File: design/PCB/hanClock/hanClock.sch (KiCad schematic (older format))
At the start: 36 parts

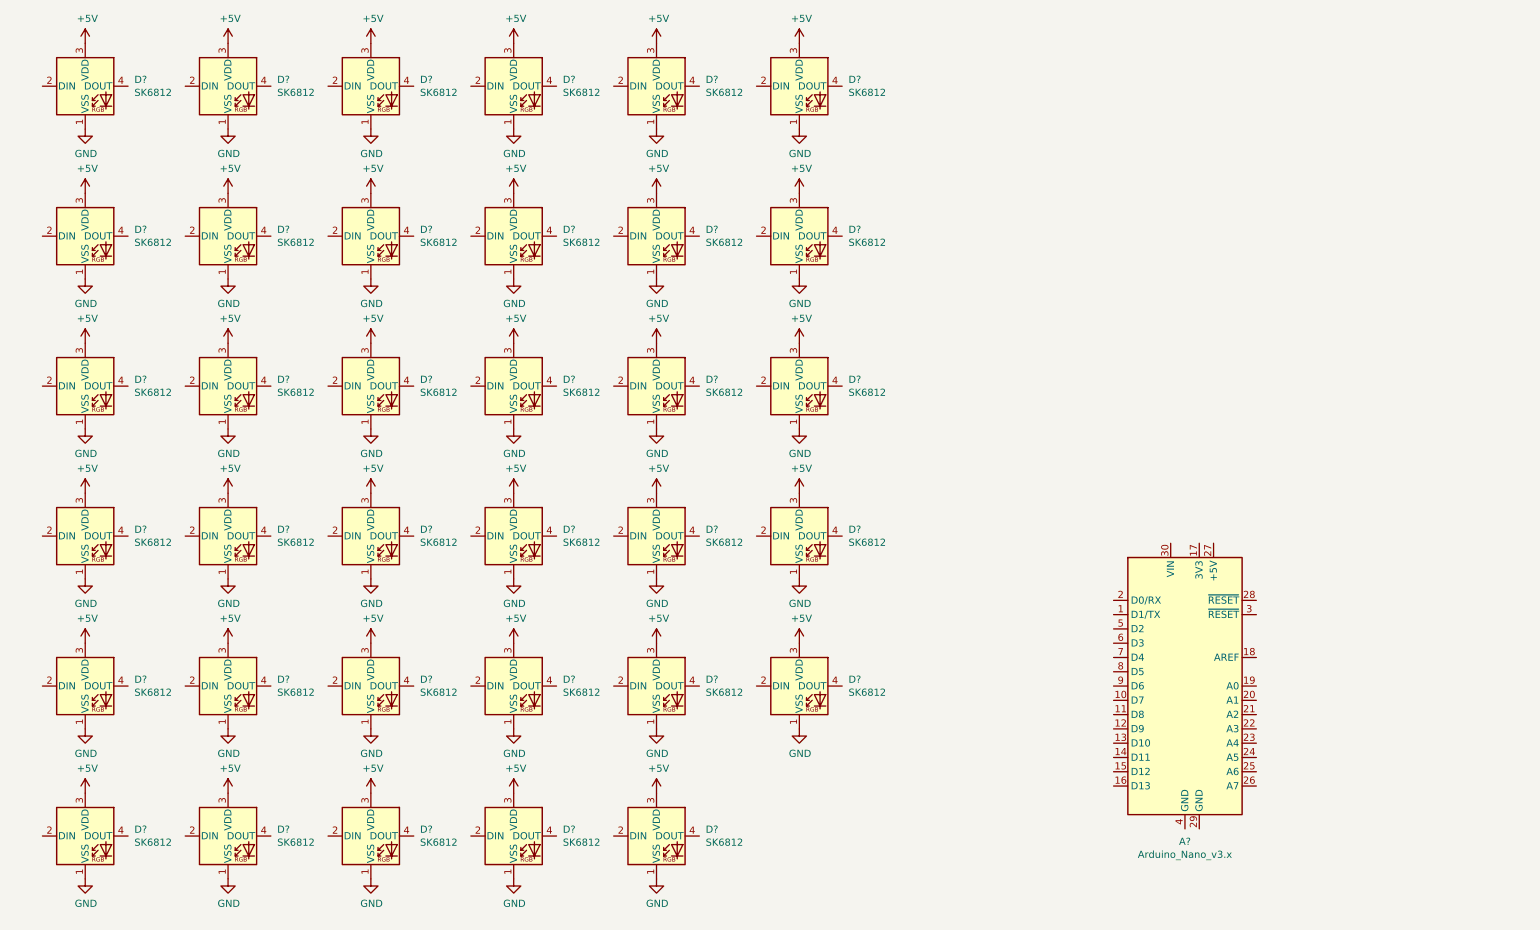
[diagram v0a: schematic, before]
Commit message: Finished design 커밋을 안 한 한참동안 PCB 다 만들고 외부 디자인도 다 해서 파일을 이렇게 저장했다.
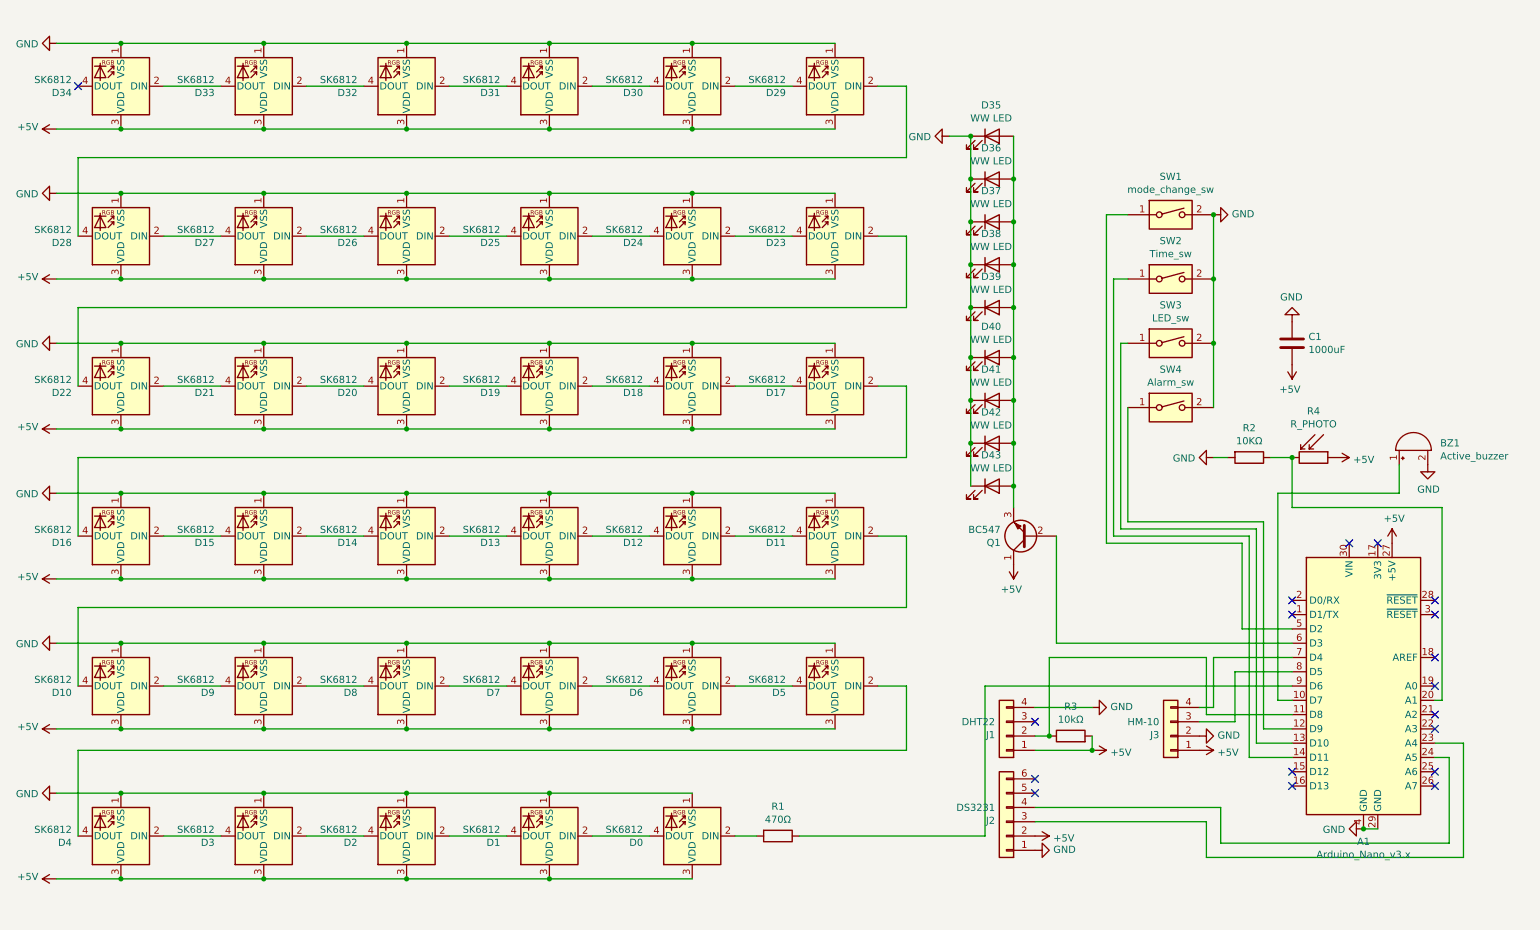
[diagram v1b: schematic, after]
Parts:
- added BZ1: Active_buzzer, parts:buzzer, symbol Device:Buzzer
- added C1: 1000uF, parts:C_K14, symbol Device:C
- added D35, D36, D37, D38, D39, D40, D41, D42, D43: WW LED, parts:3216LED, symbol Device:LED
- added J1: DHT22, parts:PinSocket_1x04_P2.54mm_Horizontal, symbol Connector_Generic:Conn_01x04
- added J2: DS3231, parts:PinSocket_1x06_P2.54mm_Horizontal, symbol Connector_Generic:Conn_01x06
- added J3: HM-10, Connector_PinSocket_2.54mm:PinSocket_1x04_P2.54mm_Vertical, symbol Connector_Generic:Conn_01x04
- added Q1: BC547, parts:BC547, symbol Device:Q_NPN_CBE
- added R1: 470Ω, Resistor_THT:R_Axial_DIN0207_L6.3mm_D2.5mm_P10.16mm_Horizontal, symbol Device:R
- added R2: 10KΩ, Resistor_THT:R_Axial_DIN0207_L6.3mm_D2.5mm_P10.16mm_Horizontal, symbol Device:R
- added R3: 10kΩ, Resistor_THT:R_Axial_DIN0207_L6.3mm_D2.5mm_P10.16mm_Horizontal, symbol Device:R
- added R4: R_PHOTO, Resistor_THT:R_Axial_DIN0204_L3.6mm_D1.6mm_P2.54mm_Vertical, symbol Device:R_PHOTO
- added SW1: mode_change_sw, parts:SMDbutton, symbol Switch:SW_DIP_x01
- added SW2: Time_sw, parts:KLT_SW, symbol Switch:SW_DIP_x01
- added SW3: LED_sw, parts:KLT_SW, symbol Switch:SW_DIP_x01
- added SW4: Alarm_sw, parts:KLT_SW, symbol Switch:SW_DIP_x01
- D0, D1, D10, D11, D12, D13, D14, D15, D16, D17, D18, D19, D2, D20, D21, D22, D23, D24, D25, D26, D27, D28, D29, D3, D30, D31, D32, D33, D34, D4, D5, D6, D7, D8, D9: renamed from D?; footprint LED_SMD:LED_SK6812_PLCC4_5.0x5.0mm_P3.2mm -> parts:LED_SK6812_PLCC4_5.0x5.0mm_P3.2mm
- gave numbers to parts that had none: 1
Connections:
- net +5V: now also A1.27 (+5V), C1.2, J1.1 (Pin_1), J2.2 (Pin_2), J3.1 (Pin_1), Q1.1 (C), R3.2, R4.1
- net GND: now also A1.29 (GND), A1.4 (GND), BZ1.2 (+), C1.1, D35.1 (K), D36.1 (K), D37.1 (K), D38.1 (K), D39.1 (K), D40.1 (K), D41.1 (K), D42.1 (K), D43.1 (K), J1.4 (Pin_4), J2.1 (Pin_1), J3.2 (Pin_2), R2.2, SW1.2, SW2.2, SW3.2, SW4.2
- net at D0.2 (DIN): now also R1.2
- net at D0.4 (DOUT): now also D1.2 (DIN)
- net at D34.2 (DIN): now also D33.4 (DOUT)
- net at D6.2 (DIN): now also D5.4 (DOUT)
- net at D6.4 (DOUT): now also D7.2 (DIN)
- net at D5.2 (DIN): now also D4.4 (DOUT)
- net at D2.2 (DIN): now also D1.4 (DOUT)
- net at D2.4 (DOUT): now also D3.2 (DIN)
- net at D8.2 (DIN): now also D7.4 (DOUT)
- net at D8.4 (DOUT): now also D9.2 (DIN)
- net at D12.2 (DIN): now also D11.4 (DOUT)
- net at D12.4 (DOUT): now also D13.2 (DIN)
- net at D11.2 (DIN): now also D10.4 (DOUT)
- net at D18.2 (DIN): now also D17.4 (DOUT)
- net at D18.4 (DOUT): now also D19.2 (DIN)
- net at D17.2 (DIN): now also D16.4 (DOUT)
- net at D14.2 (DIN): now also D13.4 (DOUT)
- net at D14.4 (DOUT): now also D15.2 (DIN)
- net at D20.2 (DIN): now also D19.4 (DOUT)
- net at D20.4 (DOUT): now also D21.2 (DIN)
- net at D24.2 (DIN): now also D23.4 (DOUT)
- net at D24.4 (DOUT): now also D25.2 (DIN)
- net at D23.2 (DIN): now also D22.4 (DOUT)
- net at D30.2 (DIN): now also D29.4 (DOUT)
- net at D30.4 (DOUT): now also D31.2 (DIN)
- net at D29.2 (DIN): now also D28.4 (DOUT)
- net at D26.2 (DIN): now also D25.4 (DOUT)
- net at D26.4 (DOUT): now also D27.2 (DIN)
- net at D32.2 (DIN): now also D31.4 (DOUT)
- net at D32.4 (DOUT): now also D33.2 (DIN)
- net at D4.2 (DIN): now also D3.4 (DOUT)
- net at D10.2 (DIN): now also D9.4 (DOUT)
- net at D16.2 (DIN): now also D15.4 (DOUT)
- net at D22.2 (DIN): now also D21.4 (DOUT)
- net at D28.2 (DIN): now also D27.4 (DOUT)
- net at A1.10 (D7): now also BZ1.1 (-)
- net at A1.11 (D8): now also J1.2 (Pin_2), R3.1
- net at A1.12 (D9): now also SW4.1
- net at A1.13 (D10): now also SW3.1
- net at A1.14 (D11): now also SW2.1
- net at A1.20 (A1): now also R2.1, R4.2
- net at A1.23 (A4): now also J2.3 (Pin_3)
- net at A1.24 (A5): now also J2.4 (Pin_4)
- net at A1.5 (D2): now also SW1.1
- net at A1.6 (D3): now also Q1.2 (B)
- net at A1.7 (D4): now also J3.4 (Pin_4)
- net at A1.8 (D5): now also J3.3 (Pin_3)
- net at A1.9 (D6): now also R1.1
- new net: D35.2 (A), D36.2 (A), D37.2 (A), D38.2 (A), D39.2 (A), D40.2 (A), D41.2 (A), D42.2 (A), D43.2 (A), Q1.3 (E)
- no-connect marks 0 -> 18
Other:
- moved on the sheet: A1, D0, D1, D10, D11, D12, D13, D14, D15, D16, D17, D18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

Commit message: PCB디자인 하는 중
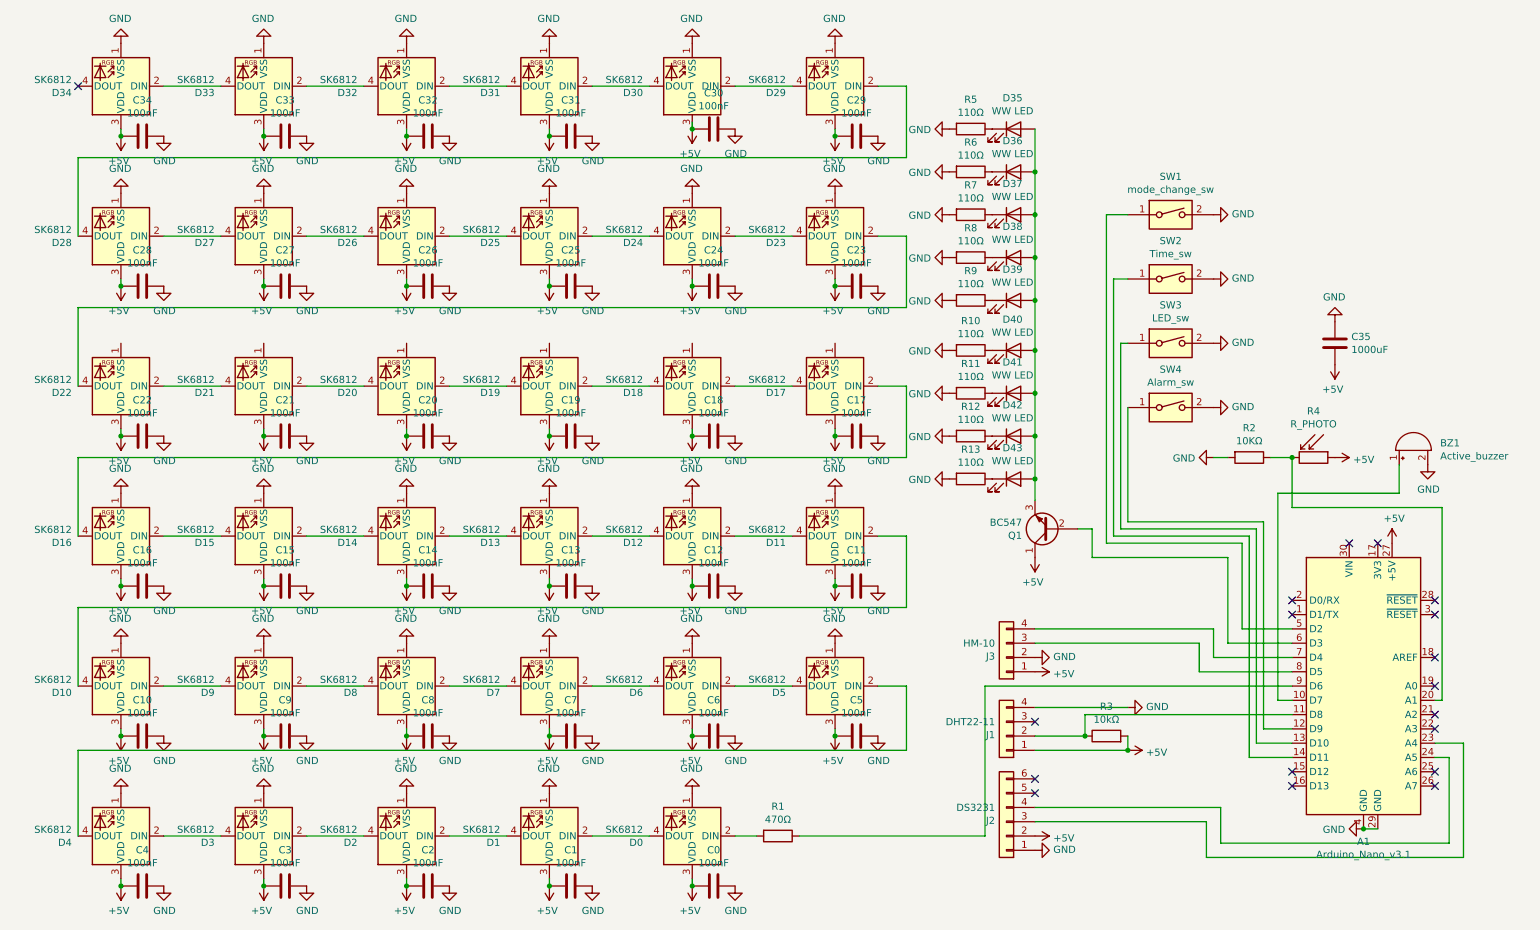
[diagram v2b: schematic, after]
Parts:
- added C0, C1, C10, C11, C12, C13, C14, C15, C16, C17, C18, C19, C2, C20, C21, C22, C23, C24, C25, C26, C27, C28, C29, C3, C30, C31, C32, C33, C34, C4, C5, C6, C7, C8, C9: 100nF, Capacitor_SMD:C_1206_3216Metric_Pad1.33x1.80mm_HandSolder, symbol Device:C
- added R10, R11, R12, R13, R5, R6, R7, R8, R9: 110Ω, Resistor_SMD:R_1206_3216Metric_Pad1.30x1.75mm_HandSolder, symbol Device:R
- A1: value Arduino_Nano_v3.x -> Arduino_Nano_v3.1
- D0, D1, D10, D11, D12, D13, D14, D15, D16, D17, D18, D19, D2, D20, D21, D22, D23, D24, D25, D26, D27, D28, D29, D3, D30, D31, D32, D33, D34, D4, D5, D6, D7, D8, D9: footprint parts:LED_SK6812_PLCC4_5.0x5.0mm_P3.2mm -> LED_SMD:LED_SK6812_PLCC4_5.0x5.0mm_P3.2mm
- D35, D36, D37, D38, D39, D40, D41, D42, D43: footprint parts:3216LED -> LED_SMD:LED_1206_3216Metric_Pad1.42x1.75mm_HandSolder
- J1: value DHT22 -> DHT22-11; footprint parts:PinSocket_1x04_P2.54mm_Horizontal -> Connector_PinSocket_2.54mm:PinSocket_1x04_P2.54mm_Vertical
- J2: footprint parts:PinSocket_1x06_P2.54mm_Horizontal -> Connector_PinSocket_2.54mm:PinSocket_1x06_P2.54mm_Vertical
- renumbered C1 to C35
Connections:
- net +5V: now also C0.2, C1.2, C10.2, C11.2, C12.2, C13.2, C14.2, C15.2, C16.2, C17.2, C18.2, C19.2, C2.2, C20.2, C21.2, C22.2, C23.2, C24.2, C25.2, C26.2, C27.2, C28.2, C29.2, C3.2, C30.2, C31.2, C32.2, C33.2, C34.2, C4.2, C5.2, C6.2, C7.2, C8.2, C9.2
- net GND: now also C0.1, C1.1, C10.1, C11.1, C12.1, C13.1, C14.1, C15.1, C16.1, C17.1, C18.1, C19.1, C2.1, C20.1, C21.1, C22.1, C23.1, C24.1, C25.1, C26.1, C27.1, C28.1, C29.1, C3.1, C30.1, C31.1, C32.1, C33.1, C34.1, C4.1, C5.1, C6.1, C7.1, C8.1, C9.1, R10.2, R11.2, R12.2, R13.2, R5.2, R6.2, R7.2, R8.2, R9.2; no longer D17.1 (VSS), D18.1 (VSS), D19.1 (VSS), D20.1 (VSS), D21.1 (VSS), D22.1 (VSS), D35.1 (K), D36.1 (K), D37.1 (K), D38.1 (K), D39.1 (K), D40.1 (K), D41.1 (K), D42.1 (K), D43.1 (K)
- new net: D36.1 (K), R6.1
- new net: D37.1 (K), R7.1
- new net: D38.1 (K), R8.1
- new net: D39.1 (K), R9.1
- new net: D40.1 (K), R10.1
- new net: D41.1 (K), R11.1
- new net: D42.1 (K), R12.1
- new net: D43.1 (K), R13.1
- new net: D35.1 (K), R5.1
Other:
- moved on the sheet: C35, D35, D36, D37, D38, D39, D40, D41, D42, D43, J3, Q1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
